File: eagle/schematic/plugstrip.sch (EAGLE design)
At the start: 31 parts, among them U1 Hall Effect, U2 Current ADC, U3 Voltage ADC

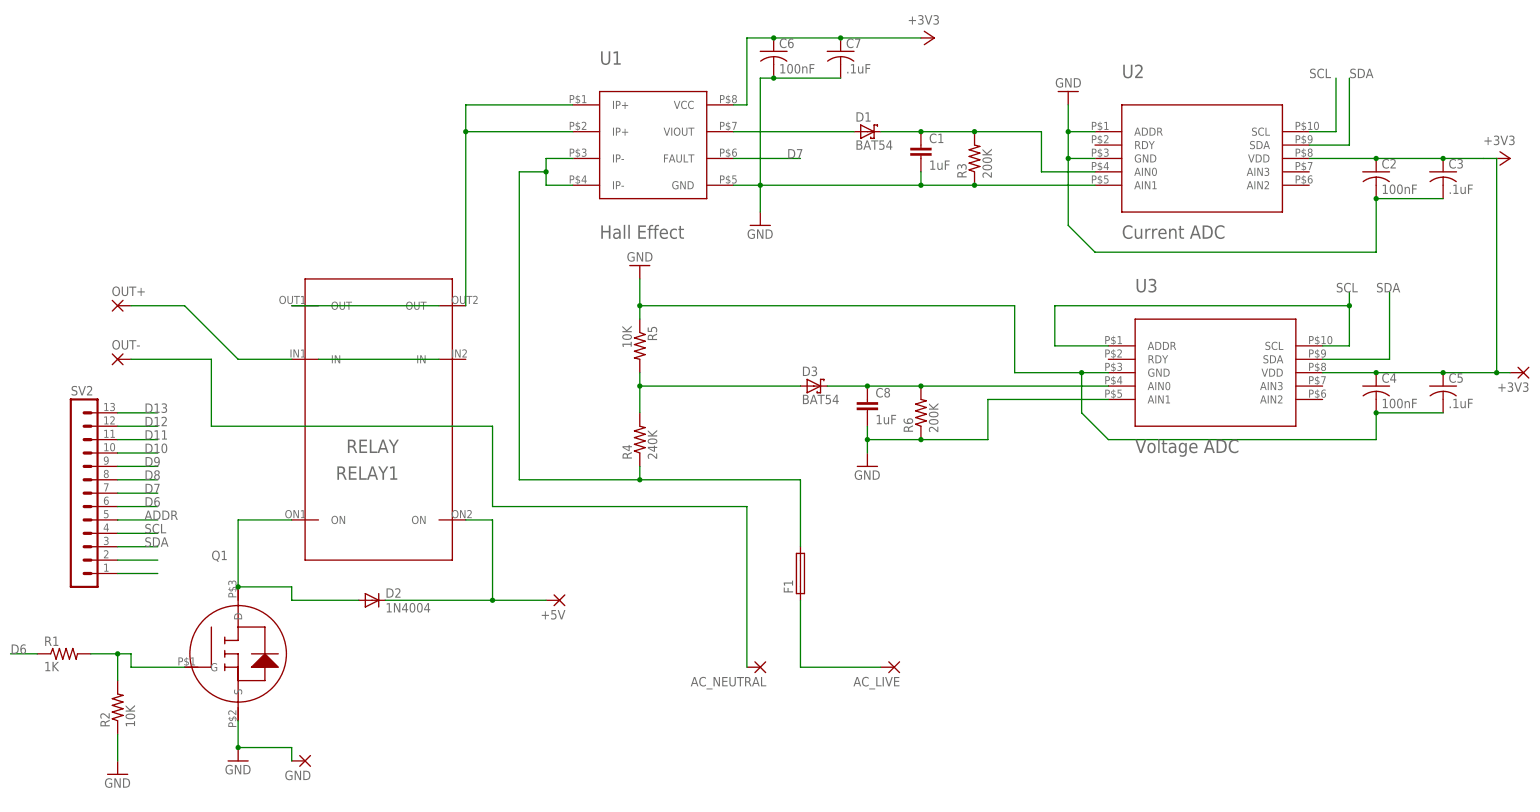
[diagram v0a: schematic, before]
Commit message: layout!
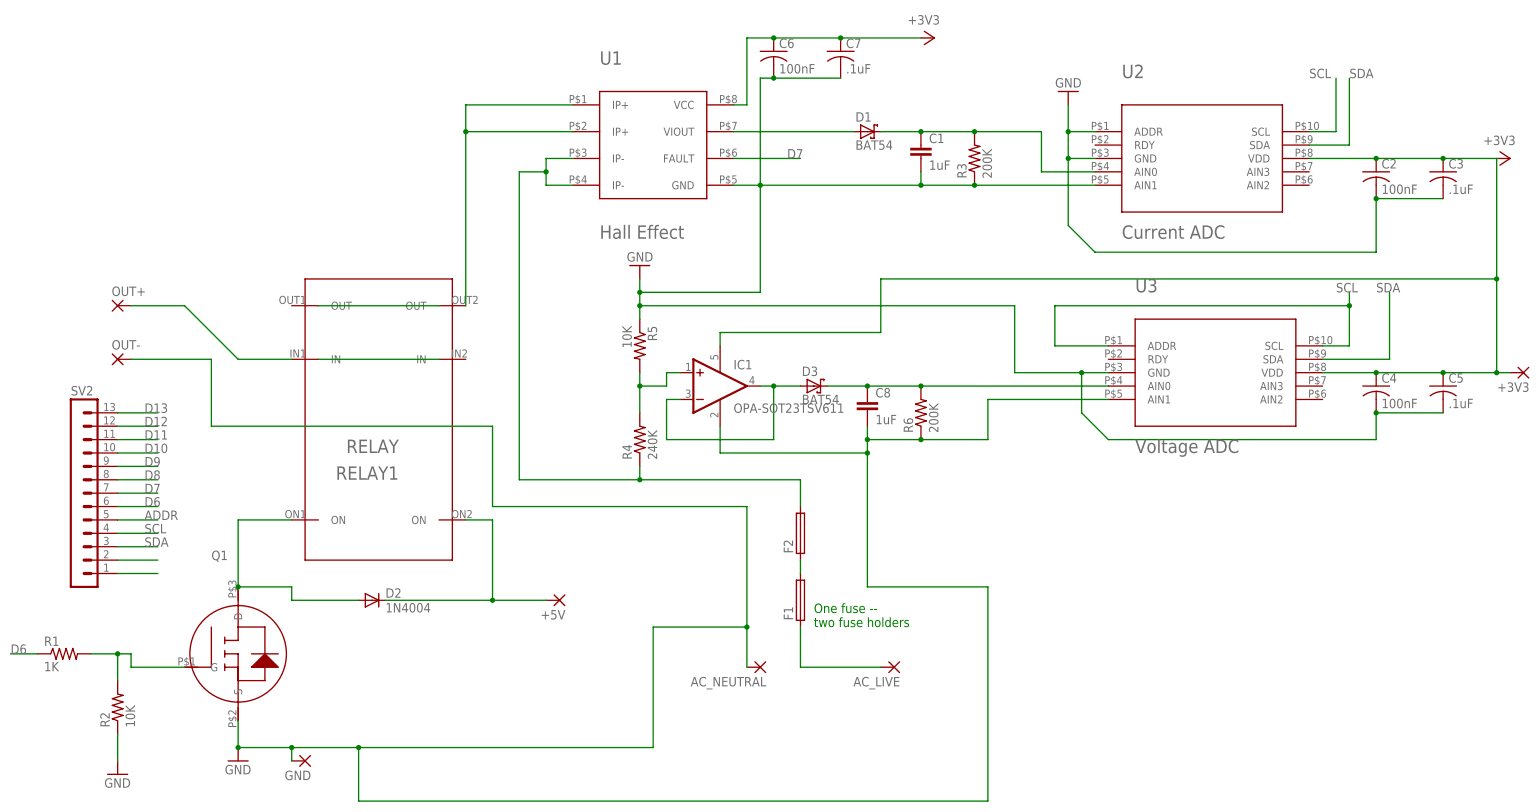
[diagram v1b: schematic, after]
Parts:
- added F2: (no value), fuse:19560
- added IC1: OPA-SOT23TSV611, linear:OPA-SOT23TSV611
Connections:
- removed net AC_NEUTRAL: AC_NEUTRAL.P, OUT-.P
- removed net N$2: RELAY1.OUT@1
- new net N$17: D3.A, IC1.-IN, IC1.OUT
- new net N$3: F1.2, F2.1
- net +3V3: now also IC1.V+
- net AC_LIVE: now also F2.2; no longer F1.2
- net GND: now also AC_NEUTRAL.P, IC1.V-, OUT-.P
- net N$31: now also IC1.+IN; no longer D3.A
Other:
- note added: "One fuse -- two fuse holders"
- moved on the sheet: F1
